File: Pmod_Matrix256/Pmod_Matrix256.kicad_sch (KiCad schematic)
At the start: 1 part, among them U1 OSLB56317-ARA

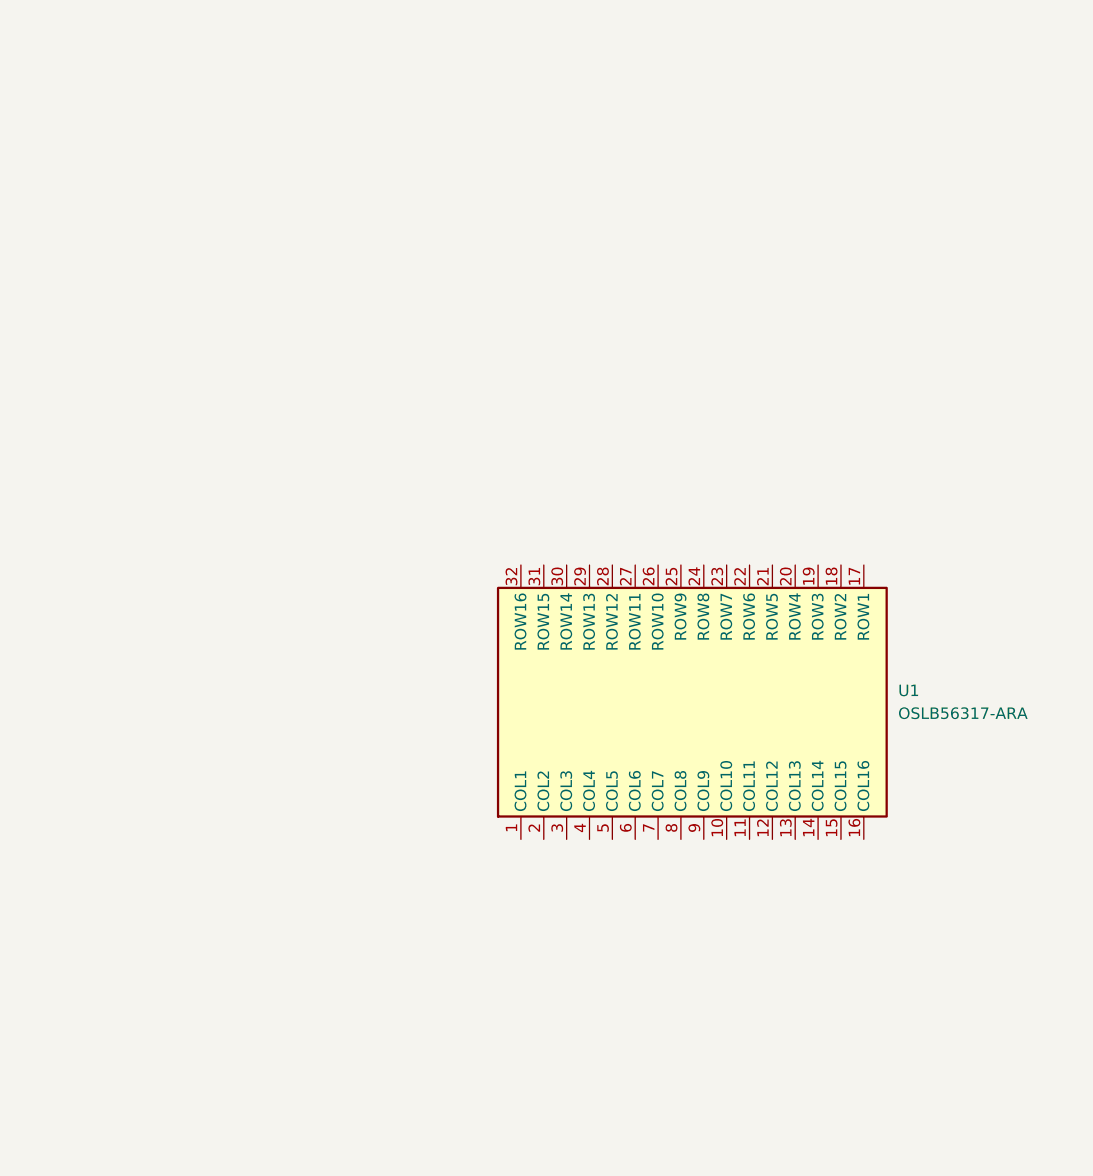
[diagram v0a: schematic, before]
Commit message: 0811
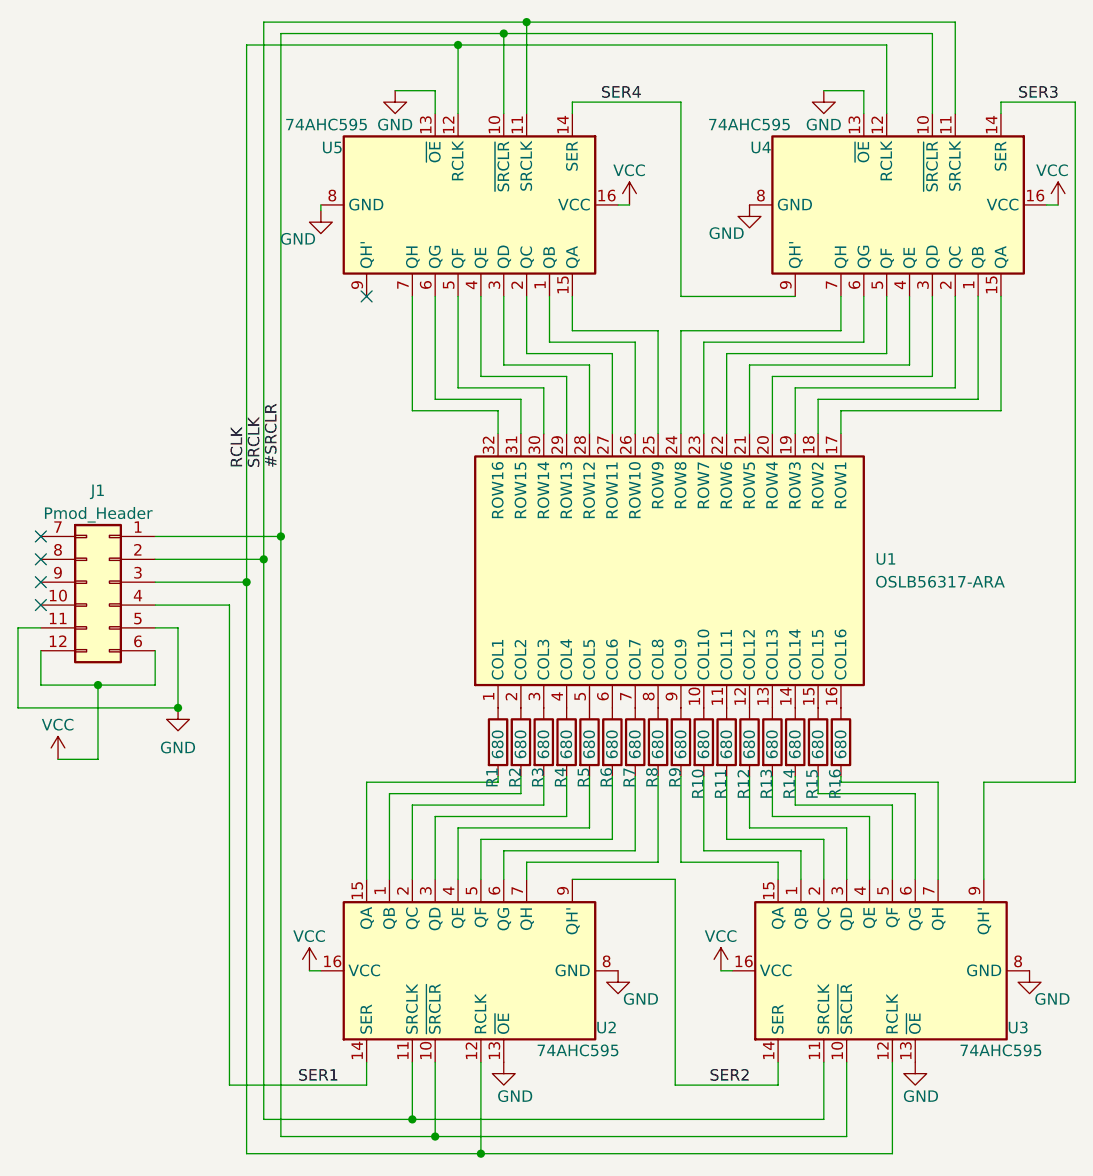
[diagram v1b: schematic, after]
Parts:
- added J1: Pmod_Header, MyLibrary:Pmod, symbol MyLibrary:Pmod_Header
- added R1, R10, R11, R12, R13, R14, R15, R16, R2, R3, R4, R5, R6, R7, R8, R9: 680, Resistor_SMD:R_0603_1608Metric_Pad0.98x0.95mm_HandSolder, symbol Device:R
- added U2, U3, U4, U5: 74AHC595, Package_SO:SOIC-16_3.9x9.9mm_P1.27mm, symbol 74xx:74AHC595
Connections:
- net at U1.1 (COL1): now also R1.1
- net at U1.10 (COL10): now also R10.1
- net at U1.11 (COL11): now also R11.1
- net at U1.12 (COL12): now also R12.1
- net at U1.13 (COL13): now also R13.1
- net at U1.14 (COL14): now also R14.1
- net at U1.15 (COL15): now also R15.1
- net at U1.16 (COL16): now also R16.1
- net at U1.17 (ROW1): now also U4.15 (QA)
- net at U1.18 (ROW2): now also U4.1 (QB)
- net at U1.19 (ROW3): now also U4.2 (QC)
- net at U1.2 (COL2): now also R2.1
- net at U1.20 (ROW4): now also U4.3 (QD)
- net at U1.21 (ROW5): now also U4.4 (QE)
- net at U1.22 (ROW6): now also U4.5 (QF)
- net at U1.23 (ROW7): now also U4.6 (QG)
- net at U1.24 (ROW8): now also U4.7 (QH)
- net at U1.25 (ROW9): now also U5.15 (QA)
- net at U1.26 (ROW10): now also U5.1 (QB)
- net at U1.27 (ROW11): now also U5.2 (QC)
- net at U1.28 (ROW12): now also U5.3 (QD)
- net at U1.29 (ROW13): now also U5.4 (QE)
- net at U1.3 (COL3): now also R3.1
- net at U1.30 (ROW14): now also U5.5 (QF)
- net at U1.31 (ROW15): now also U5.6 (QG)
- net at U1.32 (ROW16): now also U5.7 (QH)
- net at U1.4 (COL4): now also R4.1
- net at U1.5 (COL5): now also R5.1
- net at U1.6 (COL6): now also R6.1
- net at U1.7 (COL7): now also R7.1
- net at U1.8 (COL8): now also R8.1
- net at U1.9 (COL9): now also R9.1
- new net: R10.2, U3.1 (QB)
- new net: R7.2, U2.6 (QG)
- new net: R2.2, U2.1 (QB)
- new net: R12.2, U3.3 (QD)
- new net: R3.2, U2.2 (QC)
- new net: R13.2, U3.4 (QE)
- new net: R1.2, U2.15 (QA)
- new net: R4.2, U2.3 (QD)
- new net: R5.2, U2.4 (QE)
- new net: R6.2, U2.5 (QF)
- new net: R8.2, U2.7 (QH)
- new net: R14.2, U3.5 (QF)
- new net: R15.2, U3.6 (QG)
- new net: R16.2, U3.7 (QH)
- new net: R9.2, U3.15 (QA)
- new net: R11.2, U3.2 (QC)
- new net #SRCLR: J1.1 (Pin_1), U2.10 (~{SRCLR}), U3.10 (~{SRCLR}), U4.10 (~{SRCLR}), U5.10 (~{SRCLR})
- new net GND: J1.11 (Pin_11), J1.5 (Pin_5), U2.13 (~{OE}), U2.8 (GND), U3.13 (~{OE}), U3.8 (GND), U4.13 (~{OE}), U4.8 (GND), U5.13 (~{OE}), U5.8 (GND)
- new net RCLK: J1.3 (Pin_3), U2.12 (RCLK), U3.12 (RCLK), U4.12 (RCLK), U5.12 (RCLK)
- new net SER1: J1.4 (Pin_4), U2.14 (SER)
- new net SER2: U2.9 (QH'), U3.14 (SER)
- new net SER3: U3.9 (QH'), U4.14 (SER)
- new net SER4: U4.9 (QH'), U5.14 (SER)
- new net SRCLK: J1.2 (Pin_2), U2.11 (SRCLK), U3.11 (SRCLK), U4.11 (SRCLK), U5.11 (SRCLK)
- new net VCC: J1.12 (Pin_12), J1.6 (Pin_6), U2.16 (VCC), U3.16 (VCC), U4.16 (VCC), U5.16 (VCC)
- no-connect marks 0 -> 5
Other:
- moved on the sheet: U1
